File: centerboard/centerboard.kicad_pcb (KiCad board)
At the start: 2 copper layers, 231 x 32 mm, 72 parts, among them SW1 SW_Push, U1 ProMicro

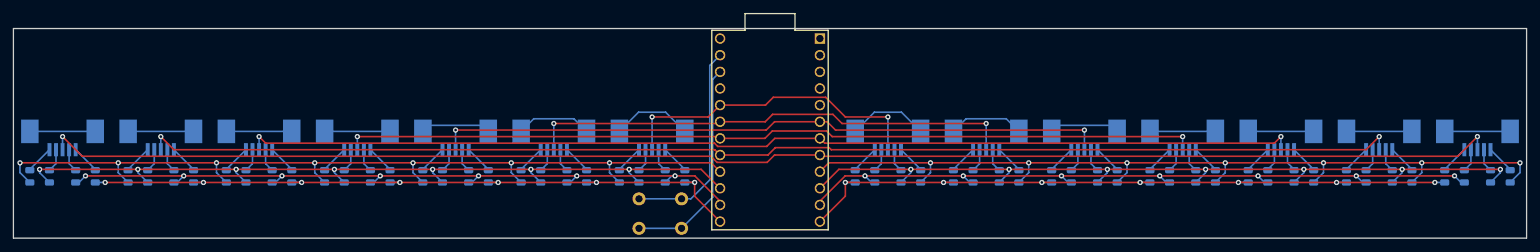
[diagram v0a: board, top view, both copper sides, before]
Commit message: centerboard redone, in 1.0 form I think
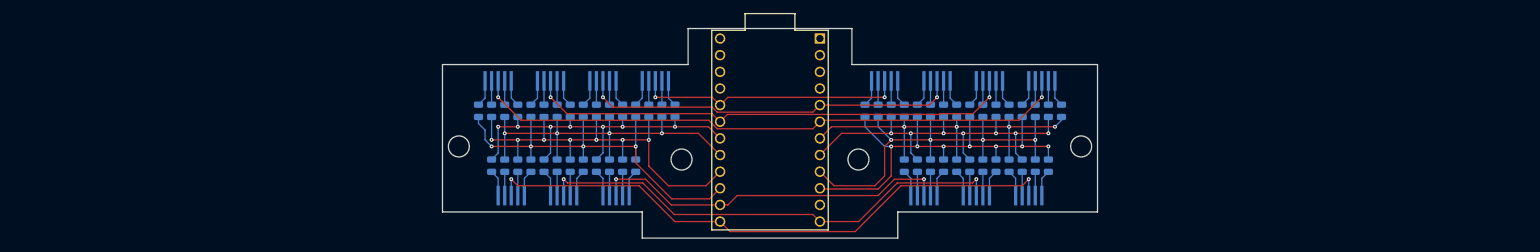
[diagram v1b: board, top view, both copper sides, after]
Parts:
- removed the D13 at (223.0, 48.1)
- removed the D14 at (220.0, 48.1)
- removed the D15 at (216.0, 48.1)
- removed the D16 at (213.0, 48.1)
- removed the D21 at (193.0, 48.1)
- removed the D22 at (190.0, 48.1)
- removed the D23 at (186.0, 48.1)
- removed the D24 at (183.0, 48.1)
- removed the D5 at (253.0, 48.1)
- removed the D56 at (42.0, 48.1)
- removed the D6 at (250.0, 48.1)
- removed the D7 at (246.0, 48.1)
- removed SW1: SW_Push, Button_Switch_THT:SW_PUSH_6mm
- added D33: 1N4148W, Diode_SMD:D_0805_2012Metric, B.Cu at (183.5, 38.1)
- added D34: 1N4148W, Diode_SMD:D_0805_2012Metric, B.Cu at (181.5, 38.1)
- added D35: 1N4148W, Diode_SMD:D_0805_2012Metric, B.Cu at (179.5, 38.1)
- added D36: 1N4148W, Diode_SMD:D_0805_2012Metric, B.Cu at (177.5, 38.1)
- added D41: 1N4148W, Diode_SMD:D_0805_2012Metric, B.Cu at (175.5, 46.4)
- added D42: 1N4148W, Diode_SMD:D_0805_2012Metric, B.Cu at (177.5, 46.4)
- added D43: 1N4148W, Diode_SMD:D_0805_2012Metric, B.Cu at (179.5, 46.4)
- added D44: 1N4148W, Diode_SMD:D_0805_2012Metric, B.Cu at (181.5, 46.4)
- added D49: 1N4148W, Diode_SMD:D_0805_2012Metric, B.Cu at (175.5, 38.1)
- added D50: 1N4148W, Diode_SMD:D_0805_2012Metric, B.Cu at (173.5, 38.1)
- added D51: 1N4148W, Diode_SMD:D_0805_2012Metric, B.Cu at (171.5, 38.1)
- added D52: 1N4148W, Diode_SMD:D_0805_2012Metric, B.Cu at (169.5, 38.1)
- added REF**: MountingHole_3.2mm_M3, MountingHole:MountingHole_3.2mm_M3, F.Cu at (168.5, 45.5)
- added REF**: MountingHole_3.2mm_M3, MountingHole:MountingHole_3.2mm_M3, F.Cu at (141.5, 45.5)
- added REF**: MountingHole_3.2mm_M3, MountingHole:MountingHole_3.2mm_M3, F.Cu at (107.5, 43.5)
- added REF**: MountingHole_3.2mm_M3, MountingHole:MountingHole_3.2mm_M3, F.Cu at (202.5, 43.5)
- JC_L1, JC_L2, JC_L3, JC_L4, JC_L5, JC_L6, JC_L7, JC_R1, JC_R2, JC_R3, JC_R4, JC_R5, JC_R6, JC_R7: footprint Connector_FFC-FPC:TE_84952-5_1x05-1MP_P1.0mm_Horizontal -> panelization:FFC clamp fit 1x05 1.00mm
- moved D8 132.9 mm to (110.5, 38.1)
- moved D1 69.2 mm to (199.5, 38.1)
- moved D2 68.2 mm to (197.5, 38.1)
- moved D7 68.2 mm to (112.5, 38.1)
- moved JC_L1 67.1 mm to (196.5, 33.5), turned to 180 degrees
- moved JC_R1 67.1 mm to (113.5, 33.5), turned to 180 degrees
- moved D3 66.3 mm to (195.5, 38.1)
- moved D6 66.3 mm to (114.5, 38.1)
- moved D4 65.3 mm to (193.5, 38.1)
- moved D5 65.3 mm to (116.5, 38.1)
- moved D16 61.5 mm to (118.5, 46.4), turned to -90 degrees
- moved D15 56.5 mm to (116.5, 46.4), turned to -90 degrees
- moved JC_L2 54.2 mm to (194.5, 51.0)
- moved JC_R2 54.2 mm to (115.5, 51.0)
- moved D14 50.5 mm to (114.5, 46.4), turned to -90 degrees
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- renumbered D49 to D13, D50 to D14, D51 to D15, D52 to D16, D45 to D21, D46 to D22, D47 to D23, D48 to D24, D41 to D29, D42 to D30, D43 to D31, D44 to D32, D33 to D45, D34 to D46, D35 to D47, D36 to D48, D53 to D5, D29 to D53, D30 to D54, D31 to D55, D32 to D56, D54 to D6, D55 to D7
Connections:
- D10 pad 2: Net-(D18-A) -> Net-(D10-A)
- D11 pad 2: Net-(D19-A) -> Net-(D11-A)
- D12 pad 2: Net-(D20-A) -> Net-(D12-A)
- D17 pad 2: Net-(D33-A) -> Net-(D17-A)
- D18 pad 2: Net-(D34-A) -> Net-(D18-A)
- D19 pad 2: Net-(D35-A) -> Net-(D19-A)
- D20 pad 2: Net-(D36-A) -> Net-(D20-A)
- D25 pad 2: Net-(D49-A) -> Net-(D25-A)
- D26 pad 2: Net-(D50-A) -> Net-(D26-A)
- D27 pad 2: Net-(D51-A) -> Net-(D27-A)
- D28 pad 2: Net-(D52-A) -> Net-(D28-A)
- D8 pad 1: ROW_L4 -> ROW_R4
- D8 pad 2: Net-(D12-A) -> Net-(D8-A)
- D9 pad 2: Net-(D17-A) -> Net-(D9-A)
- U1 pad 10: ROW_L2 -> ROW_L4
- U1 pad 11: ROW_L3 -> unconnected-(U1-B4-Pad11)
- U1 pad 12: ROW_L4 -> COL_4
- U1 pad 13: ROW_R1 -> COL_2
- U1 pad 14: ROW_R2 -> COL_6
- U1 pad 15: ROW_R3 -> ROW_R4
- U1 pad 16: ROW_R4 -> ROW_R3
- U1 pad 17: COL_2 -> ROW_R2
- U1 pad 18: COL_4 -> ROW_R1
- U1 pad 19: COL_6 -> COL_3
- U1 pad 22: Net-(U1-RST) -> unconnected-(U1-RST-Pad22)
- U1 pad 23: Net-(SW1-Pad1) -> unconnected-(U1-GND-Pad23)
- U1 pad 5: unconnected-(U1-SDA-Pad5) -> COL_5
- U1 pad 6: COL_5 -> COL_1
- U1 pad 7: COL_3 -> ROW_L1
- U1 pad 8: COL_1 -> ROW_L2
- U1 pad 9: ROW_L1 -> ROW_L3
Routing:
- net COL_1: track 223.1 -> 91.7 mm
- net COL_2: track 192.6 -> 90.6 mm
- net COL_3: track 161.8 -> 75.1 mm
- net ROW_L1: track 132.8 -> 58.0 mm, vias 7 -> 4
- net ROW_R4: track 132.8 -> 65.2 mm, vias 7 -> 4
- net ROW_L2: track 123.4 -> 59.5 mm
- net ROW_R3: track 123.4 -> 64.0 mm
- net COL_4: track 130.6 -> 73.4 mm
- net ROW_R2: track 108.9 -> 56.3 mm, vias 7 -> 4
- net ROW_R1: track 108.1 -> 56.9 mm
- net ROW_L3: track 108.4 -> 63.1 mm, vias 7 -> 4
- net COL_5: track 103.1 -> 57.9 mm
- net ROW_L4: track 108.1 -> 66.3 mm
- net Net-(U1-RST): track 32.8 -> 0.00 mm
- net Net-(SW1-Pad1): track 31.7 -> 0.00 mm
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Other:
- board size 231 x 32 mm -> 100 x 32 mm
